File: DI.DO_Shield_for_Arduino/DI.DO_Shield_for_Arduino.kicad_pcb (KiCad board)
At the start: 2 copper layers, 83.9 x 77.7 mm, 47 parts, among them J1 CONN_08X2, J10 CONN_08X2, J2 CONN_08X2, J3 CONN_08X2, J4 CONN_08X2, J5 CONN_08X2, J6 CONN_08X2, J7 CONN_08X2, J8 CONN_08X2, J9 CONN_08X2, U1 MCP23S08, U1_A0 JUMPER-SMT_2_NC, U1_A1 JUMPER-SMT_2_NO, U1_A2 JUMPER-SMT_2_NO, U2 MCP23S08, U2_A0 JUMPER-SMT_2_NO, U2_A1 JUMPER-SMT_2_NC, U2_A2 JUMPER-SMT_2_NO

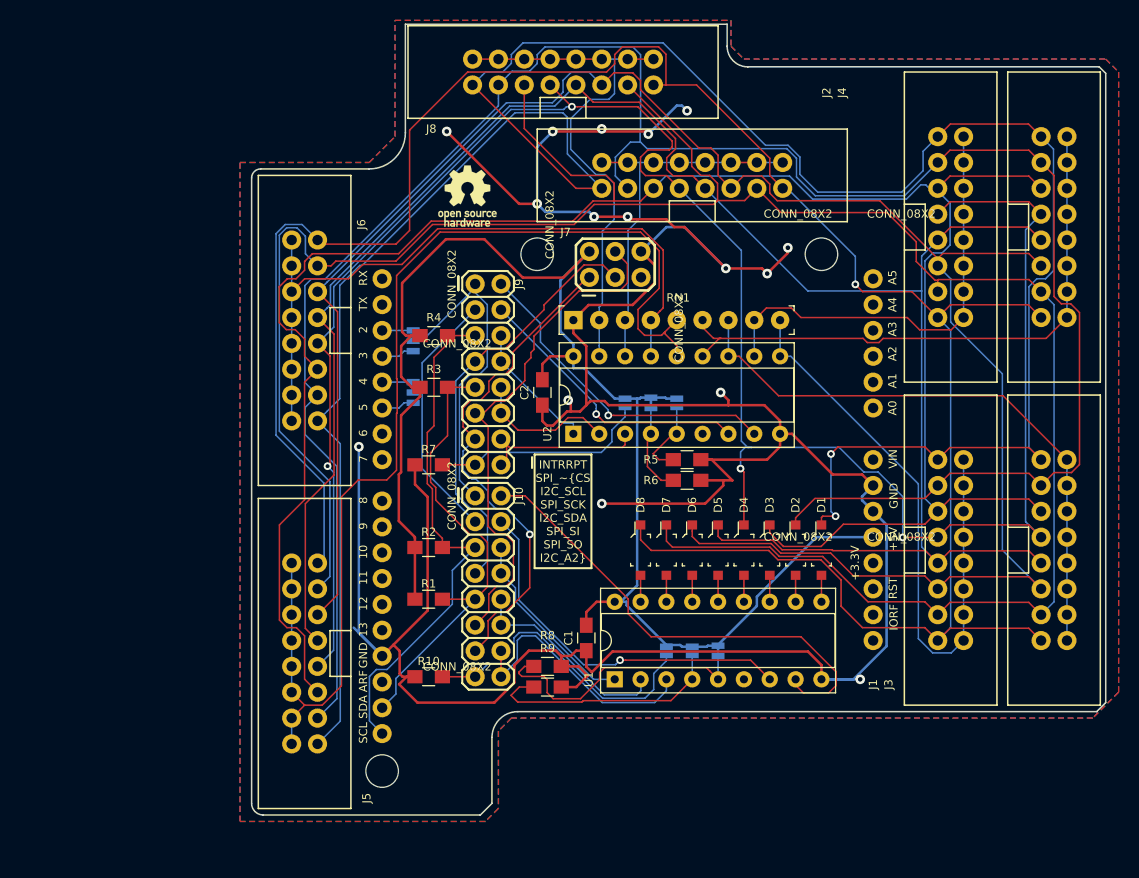
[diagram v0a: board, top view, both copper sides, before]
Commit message: add buttons and pots sub-boards, push changes
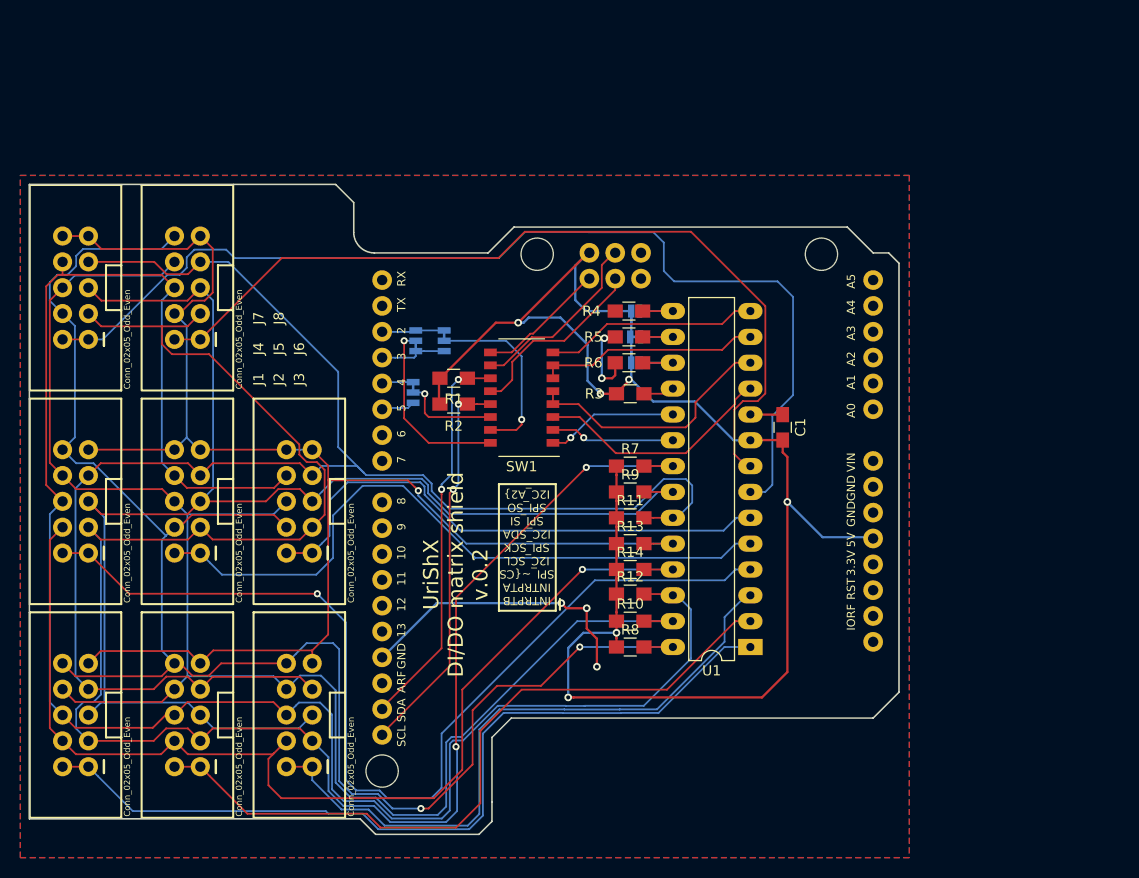
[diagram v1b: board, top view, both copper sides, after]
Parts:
- removed C2: 0.1uF, Capacitors_SMD:C_0805_HandSoldering
- removed D1, D2, D3, D4, D5, D6, D7, D8: 1N4148W-TP, digikey-footprints:SOD-123
- removed INT1: JUMPER-SMT_3_1-NC, SparkFun Jumpers:SMT-JUMPER_3_1-NC_TRACE_SILK
- removed J10, J9: CONN_08X2, SparkFun Connectors:2X8
- removed REF***: KiCad-Logo_6mm_SilkScreen, Symbols:KiCad-Logo_6mm_SilkScreen
- removed REF***: OSHW-Logo_5.7x6mm_SilkScreen, Symbols:OSHW-Logo_5.7x6mm_SilkScreen
- removed RN1: 4609X-101-103LF, digikey-footprints:SIP-9_P2.54mm
- removed U1_A0: JUMPER-SMT_2_NC, SparkFun Jumpers:SMT-JUMPER_2_NC_TRACE_SILK
- removed U1_A1, U1_A2, U2_A0: JUMPER-SMT_2_NO, SparkFun Jumpers:SMT-JUMPER_2_NO_SILK
- removed U2: MCP23S08, Housings_DIP:DIP-18_W7.62mm_Socket
- removed h1, h2, h3: >VALUE, MyFootprintLib:Arduino_3.2_connector
- added INTA1: JUMPER-SMT_3_1-NC, SparkFun Jumpers:SMT-JUMPER_3_1-NC_TRACE_SILK, B.Cu at (110.2, 77.2)
- added INTB1: JUMPER-SMT_3_1-NC, SparkFun Jumpers:SMT-JUMPER_3_1-NC_TRACE_SILK, B.Cu at (107.4, 77.2)
- added R11: 2k2, Resistors_SMD:R_0805_HandSoldering, F.Cu at (128.5, 94.6)
- added R12: 2k2, Resistors_SMD:R_0805_HandSoldering, F.Cu at (128.5, 102.1)
- added R13: 2k2, Resistors_SMD:R_0805_HandSoldering, F.Cu at (128.5, 97.2)
- added R14: 2k2, Resistors_SMD:R_0805_HandSoldering, F.Cu at (128.5, 99.7)
- added SW1: SW_DIP_x08, Buttons_Switches_SMD:SW_DIP_x8_W6.15mm_Slide_Omron_A6H, F.Cu at (117.9, 82.8)
- added U2_A3: JUMPER-SMT_2_NO, SparkFun Jumpers:SMT-JUMPER_2_NO_SILK, B.Cu at (129.0, 79.4)
- B1: footprint SparkFun Boards:UNO_R3_SHIELD_ICSP -> MyFootprintLib:ARDUINO_R3
- J1, J2, J3, J4, J5, J6, J7, J8: value CONN_08X2 -> Conn_02x05_Odd_Even; footprint MyFootprintLib:2X8_SHROUDED_PTH -> SparkFun Connectors:2X5-SHROUDED
- R10, R7, R8, R9: value 10k -> 2k2
- R3, R4: value 4.7k -> 10k
- U1: value MCP23S08 -> MCP23S17; footprint Housings_DIP:DIP-18_W7.62mm_Socket -> Housings_DIP:DIP-28_W7.62mm_LongPads
- U2_A1: value JUMPER-SMT_2_NC -> JUMPER-SMT_2_NO; footprint SparkFun Jumpers:SMT-JUMPER_2_NC_TRACE_SILK -> SparkFun Jumpers:SMT-JUMPER_2_NO_SILK
- U2_A2: value JUMPER-SMT_2_NO -> JUMPER-SMT_2_NC; footprint SparkFun Jumpers:SMT-JUMPER_2_NO_SILK -> SparkFun Jumpers:SMT-JUMPER_2_NC_TRACE_SILK
- moved J4 99.9 mm to (74.0, 93.0), turned to 180 degrees
- moved J2 89.0 mm to (85.0, 114.0), turned to 180 degrees
- moved J1 87.5 mm to (74.0, 114.0), turned to 180 degrees
- moved J3 75.9 mm to (96.0, 114.0), turned to 180 degrees
- moved J7 61.6 mm to (74.0, 72.0), turned to 180 degrees
- moved J8 42.6 mm to (85.0, 72.0), turned to 180 degrees
- moved C1 28.3 mm to (143.5, 85.7), turned to 270 degrees
- moved R1 21.9 mm to (111.2, 80.9)
- moved R9 20.8 mm to (128.5, 92.1)
- moved R10 20.6 mm to (128.5, 104.8), turned to 0 degrees
- moved R7 19.8 mm to (128.5, 89.5), turned to 0 degrees
- moved R4 19.3 mm to (128.4, 74.3)
- moved R3 19.3 mm to (128.5, 82.4), turned to 0 degrees
- moved J5 18.9 mm to (85.0, 93.0)
- moved J6 16.8 mm to (96.0, 93.0)
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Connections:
- B1 pad MISO: Net-(B1-PadMISO) -> /MISO
- B1 pad MOSI: Net-(B1-PadMOSI) -> /MOSI
- B1 pad SCK: Net-(B1-PadSCK) -> /SCK
- B1 pad SCL: Net-(B1-PadSCL) -> /SCL
- B1 pad SDA: Net-(B1-PadSDA) -> /SDA
- CS1 pad 2: Net-(CS1-Pad2) -> /CS
- J1 pad 1: Net-(D1-Pad1) -> Net-(J1-Pad1)
- J1 pad 2: Net-(J1-Pad10) -> Net-(J1-Pad1)
- J1 pad 3: Net-(D2-Pad1) -> Net-(J1-Pad3)
- J1 pad 4: Net-(J1-Pad10) -> Net-(J1-Pad4)
- J1 pad 5: Net-(D3-Pad1) -> Net-(J1-Pad5)
- J1 pad 6: Net-(J1-Pad10) -> Net-(J1-Pad6)
- J1 pad 7: Net-(D4-Pad1) -> Net-(J1-Pad7)
- J1 pad 8: Net-(J1-Pad10) -> Net-(J1-Pad8)
- J1 pad 9: Net-(D5-Pad1) -> Net-(J1-Pad9)
- J2 pad 1: Net-(D1-Pad1) -> Net-(J2-Pad1)
- J2 pad 10: Net-(J2-Pad10) -> Net-(J1-Pad10)
- J2 pad 2: Net-(J2-Pad10) -> Net-(J2-Pad1)
- J2 pad 3: Net-(D2-Pad1) -> Net-(J1-Pad3)
- J2 pad 4: Net-(J2-Pad10) -> Net-(J1-Pad4)
- J2 pad 5: Net-(D3-Pad1) -> Net-(J1-Pad5)
- J2 pad 6: Net-(J2-Pad10) -> Net-(J1-Pad6)
- J2 pad 7: Net-(D4-Pad1) -> Net-(J1-Pad7)
- J2 pad 8: Net-(J2-Pad10) -> Net-(J1-Pad8)
- J2 pad 9: Net-(D5-Pad1) -> Net-(J1-Pad9)
- J3 pad 1: Net-(D1-Pad1) -> Net-(J3-Pad1)
- J3 pad 10: Net-(J3-Pad10) -> Net-(J1-Pad10)
- J3 pad 2: Net-(J3-Pad10) -> Net-(J3-Pad1)
- J3 pad 3: Net-(D2-Pad1) -> Net-(J1-Pad3)
- J3 pad 4: Net-(J3-Pad10) -> Net-(J1-Pad4)
- J3 pad 5: Net-(D3-Pad1) -> Net-(J1-Pad5)
- J3 pad 6: Net-(J3-Pad10) -> Net-(J1-Pad6)
- J3 pad 7: Net-(D4-Pad1) -> Net-(J1-Pad7)
- J3 pad 8: Net-(J3-Pad10) -> Net-(J1-Pad8)
- J3 pad 9: Net-(D5-Pad1) -> Net-(J1-Pad9)
- J4 pad 1: Net-(D1-Pad1) -> Net-(J4-Pad1)
- J4 pad 10: Net-(J4-Pad10) -> Net-(J1-Pad10)
- J4 pad 2: Net-(J4-Pad10) -> Net-(J4-Pad1)
- J4 pad 3: Net-(D2-Pad1) -> Net-(J1-Pad3)
- J4 pad 4: Net-(J4-Pad10) -> Net-(J1-Pad4)
- J4 pad 5: Net-(D3-Pad1) -> Net-(J1-Pad5)
- J4 pad 6: Net-(J4-Pad10) -> Net-(J1-Pad6)
- J4 pad 7: Net-(D4-Pad1) -> Net-(J1-Pad7)
- J4 pad 8: Net-(J4-Pad10) -> Net-(J1-Pad8)
- J4 pad 9: Net-(D5-Pad1) -> Net-(J1-Pad9)
- J5 pad 1: Net-(D1-Pad1) -> Net-(J5-Pad1)
- J5 pad 10: Net-(J5-Pad10) -> Net-(J1-Pad9)
- J5 pad 2: Net-(J5-Pad10) -> Net-(J5-Pad1)
- J5 pad 3: Net-(D2-Pad1) -> Net-(J1-Pad3)
- J5 pad 4: Net-(J5-Pad10) -> Net-(J1-Pad10)
- J5 pad 5: Net-(D3-Pad1) -> Net-(J1-Pad5)
- J5 pad 6: Net-(J5-Pad10) -> Net-(J1-Pad8)
- J5 pad 7: Net-(D4-Pad1) -> Net-(J1-Pad7)
- J5 pad 8: Net-(J5-Pad10) -> Net-(J1-Pad6)
- J5 pad 9: Net-(D5-Pad1) -> Net-(J1-Pad9)
- J6 pad 1: Net-(D1-Pad1) -> Net-(J6-Pad1)
- J6 pad 10: Net-(J6-Pad10) -> Net-(J1-Pad9)
- J6 pad 2: Net-(J6-Pad10) -> Net-(J6-Pad1)
- J6 pad 3: Net-(D2-Pad1) -> Net-(J1-Pad3)
- J6 pad 4: Net-(J6-Pad10) -> Net-(J1-Pad10)
- J6 pad 5: Net-(D3-Pad1) -> Net-(J1-Pad5)
- J6 pad 6: Net-(J6-Pad10) -> Net-(J1-Pad8)
- J6 pad 7: Net-(D4-Pad1) -> Net-(J1-Pad7)
- J6 pad 8: Net-(J6-Pad10) -> Net-(J1-Pad6)
- J6 pad 9: Net-(D5-Pad1) -> Net-(J1-Pad9)
- J7 pad 1: Net-(D1-Pad1) -> Net-(J7-Pad1)
- J7 pad 10: Net-(J7-Pad10) -> Net-(J1-Pad9)
- J7 pad 2: Net-(J7-Pad10) -> Net-(J7-Pad1)
- J7 pad 3: Net-(D2-Pad1) -> Net-(J1-Pad3)
- J7 pad 4: Net-(J7-Pad10) -> Net-(J1-Pad10)
- J7 pad 5: Net-(D3-Pad1) -> Net-(J1-Pad5)
- J7 pad 6: Net-(J7-Pad10) -> Net-(J1-Pad8)
- J7 pad 7: Net-(D4-Pad1) -> Net-(J1-Pad7)
- J7 pad 8: Net-(J7-Pad10) -> Net-(J1-Pad6)
- J7 pad 9: Net-(D5-Pad1) -> Net-(J1-Pad9)
- J8 pad 1: Net-(D1-Pad1) -> Net-(J8-Pad1)
- J8 pad 10: Net-(J8-Pad10) -> Net-(J1-Pad10)
- J8 pad 2: Net-(J8-Pad10) -> Net-(J8-Pad1)
- J8 pad 3: Net-(D2-Pad1) -> Net-(J1-Pad3)
- J8 pad 4: Net-(J8-Pad10) -> Net-(J1-Pad9)
- J8 pad 5: Net-(D3-Pad1) -> Net-(J1-Pad5)
- J8 pad 6: Net-(J8-Pad10) -> Net-(J1-Pad6)
- J8 pad 7: Net-(D4-Pad1) -> Net-(J1-Pad7)
- J8 pad 8: Net-(J8-Pad10) -> Net-(J1-Pad8)
- J8 pad 9: Net-(D5-Pad1) -> Net-(J1-Pad9)
- R1 pad 1: Net-(B1-PadSDA) -> /SDA
- R10 pad 1: Net-(J10-Pad15) -> VCC
- R10 pad 2: GND -> Net-(J1-Pad8)
- R2 pad 1: Net-(B1-PadSCL) -> /SCL
- R3 pad 1: Net-(B1-PadSDA) -> VCC
- R3 pad 2: VCC -> Net-(R3-Pad2)
- R4 pad 1: Net-(B1-PadSCL) -> Net-(R4-Pad1)
- R4 pad 2: VCC -> GND
- R7 pad 1: Net-(J9-Pad15) -> VCC
- R7 pad 2: GND -> Net-(J1-Pad3)
- R8 pad 1: Net-(R8-Pad1) -> VCC
- R8 pad 2: GND -> Net-(J1-Pad10)
- R9 pad 1: Net-(R9-Pad1) -> VCC
- R9 pad 2: GND -> Net-(J1-Pad5)
- U1 pad 1: Net-(J10-Pad6) -> Net-(J1-Pad1)
- U1 pad 10: Net-(D1-Pad2) -> GND
- U1 pad 15: Net-(D6-Pad2) -> Net-(R4-Pad1)
- U1 pad 16: Net-(D7-Pad2) -> Net-(R5-Pad1)
- U1 pad 17: Net-(D8-Pad2) -> Net-(R6-Pad1)
- U1 pad 18: VCC -> Net-(R3-Pad2)
- U1 pad 2: Net-(J10-Pad10) -> Net-(J2-Pad1)
- U1 pad 3: Net-(J10-Pad14) -> Net-(J3-Pad1)
- U1 pad 4: Net-(R9-Pad1) -> Net-(J4-Pad1)
- U1 pad 5: Net-(R8-Pad1) -> Net-(J5-Pad1)
- U1 pad 6: (no net) -> Net-(J6-Pad1)
- U1 pad 7: Net-(J10-Pad4) -> Net-(J7-Pad1)
- U1 pad 8: Net-(J10-Pad2) -> Net-(J8-Pad1)
- U1 pad 9: GND -> VCC
- U2_A1 pad 2: Net-(R6-Pad1) -> Net-(R4-Pad1)
- U2_A2 pad 2: Net-(J9-Pad15) -> Net-(R5-Pad1)
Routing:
- net GND: track 307.9 -> 39.7 mm, vias 16 -> 5
- net Net-(D1-Pad1): track 237.5 -> 0.00 mm, vias 2 -> 0
- net Net-(D8-Pad1): track 223.2 -> 0.00 mm, vias 1 -> 0
- net Net-(D7-Pad1): track 215.5 -> 0.00 mm
- net Net-(D2-Pad1): track 214.2 -> 0.00 mm
- net Net-(D4-Pad1): track 211.3 -> 0.00 mm, vias 4 -> 0
- net Net-(D3-Pad1): track 210.6 -> 0.00 mm
- net Net-(D6-Pad1): track 201.8 -> 0.00 mm
- net Net-(D5-Pad1): track 194.7 -> 0.00 mm
- net Net-(J1-Pad6): track 0.00 -> 184.1 mm
- net Net-(J1-Pad3): track 0.00 -> 183.7 mm, vias 0 -> 2
- net Net-(J1-Pad7): track 0.00 -> 159.9 mm
- net Net-(J1-Pad8): track 0.00 -> 159.6 mm
- net Net-(J1-Pad9): track 0.00 -> 146.4 mm, vias 0 -> 1
- net Net-(J1-Pad5): track 0.00 -> 144.7 mm
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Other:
- board size 83.9 x 77.7 mm -> 85.5 x 63.9 mm
- net class Default: trace_width 0.1524 -> 0.175; via_dia 0.762 -> 0.7; via_drill 0.4064 -> 0.35
- net class pwr: trace_width 0.25 -> 0.225; via_dia 0.95 -> 0.75; via_drill 0.45 -> 0.4
- rule via_min_drill: 0.35 -> 0.3
- rule via_min_size: 0.6858 -> 0.65
- board text added: "INTRPTB INTRPTA SPI_~CS I2C_SCL SPI_SCK I2C_SDA SPI_SI SPI_SO I2C_A2"
- board text added: "UriShX DI/DO matrix shield v.0.2"
- board text removed: "INTRRPT SPI_~CS I2C_SCL SPI_SCK I2C_SDA SPI_SI SPI_SO I2C_A2"
